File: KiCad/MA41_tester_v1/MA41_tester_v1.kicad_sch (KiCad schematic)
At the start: 5 parts

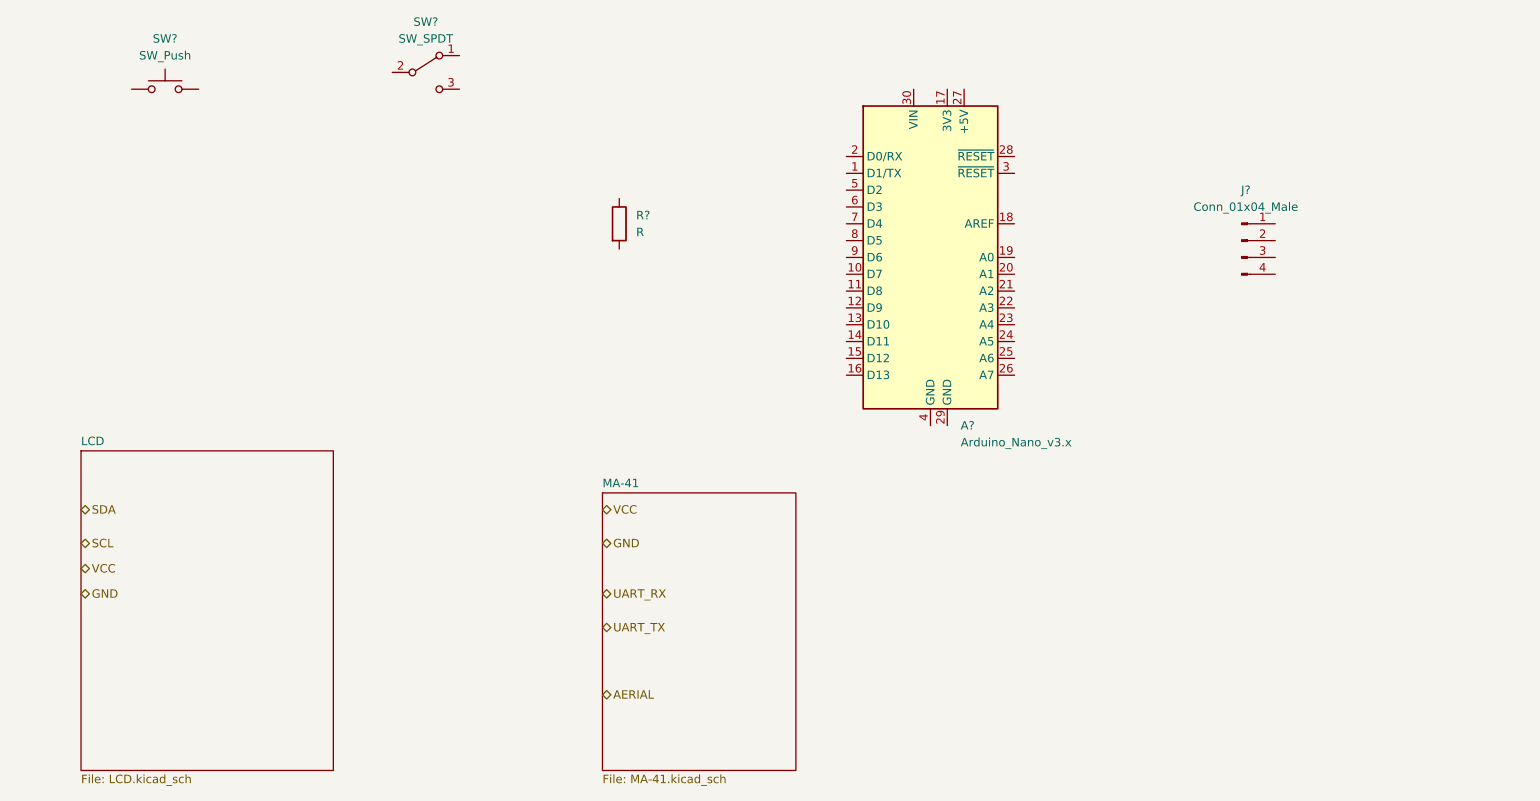
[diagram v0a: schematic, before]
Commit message: ...
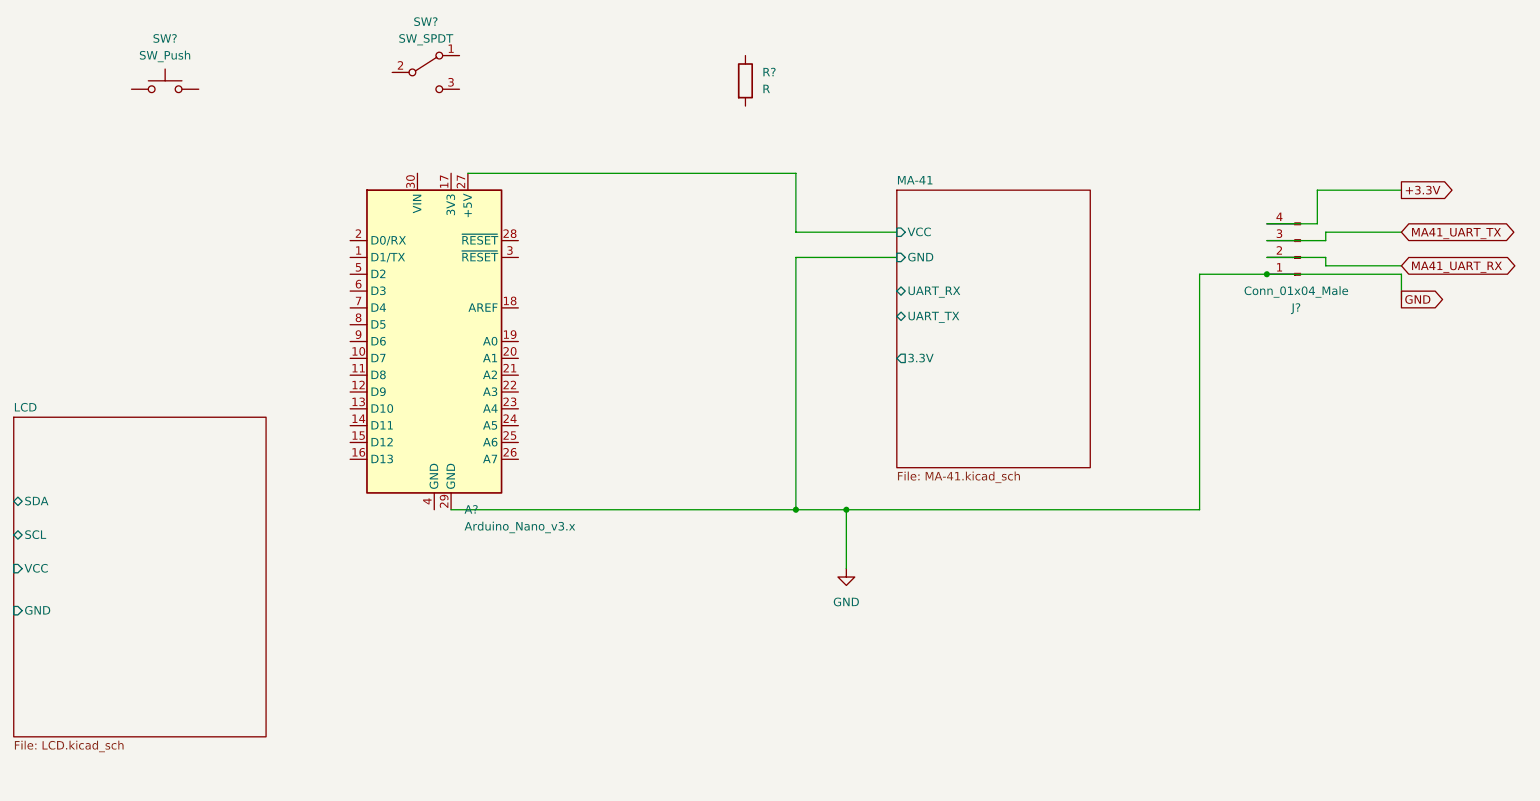
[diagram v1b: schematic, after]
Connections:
- net GND: now also A?.29 (GND), J?.1 (Pin_1)
- net MA41_UART_RX: now reaches J?.2 (Pin_2)
- net MA41_UART_TX: now reaches J?.3 (Pin_3)
- net +3.3V: now reaches J?.4 (Pin_4)
- net MA-41/VCC: now reaches A?.27 (+5V)
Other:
- sheet LCD ports: added GND, SCL, SDA, VCC; removed none
- sheet MA-41 ports: added 3.3V, GND, UART_RX, UART_TX, VCC; removed none
- moved on the sheet: A?, J?, R?
